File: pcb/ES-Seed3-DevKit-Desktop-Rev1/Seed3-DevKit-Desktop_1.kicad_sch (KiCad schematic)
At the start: 56 parts, among them J7 USB4110GFA, U12 CD4051B, U14 USBLC6-2SC6, U2 MCP6002-xSN, U4 4021, U5 4021, U6 MCP6002-xSN, U9 MCP6002-xSN

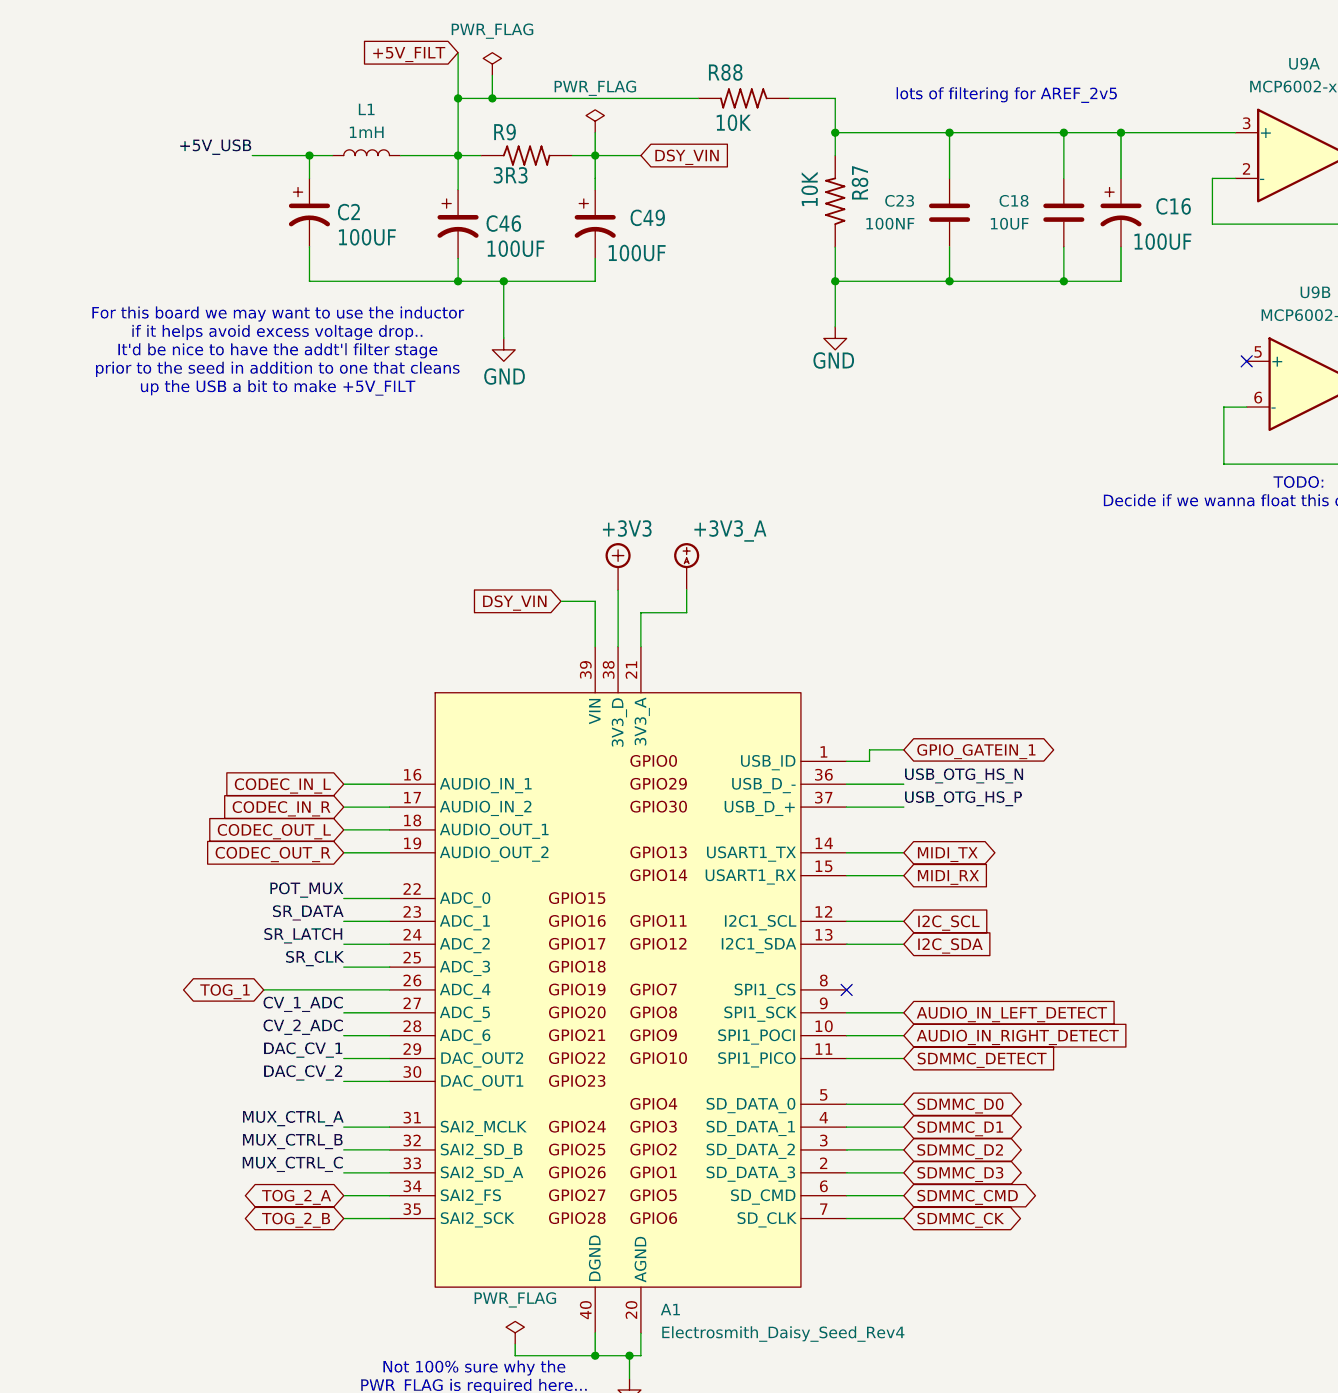
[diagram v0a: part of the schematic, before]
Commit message: routed, productions mats, etc.
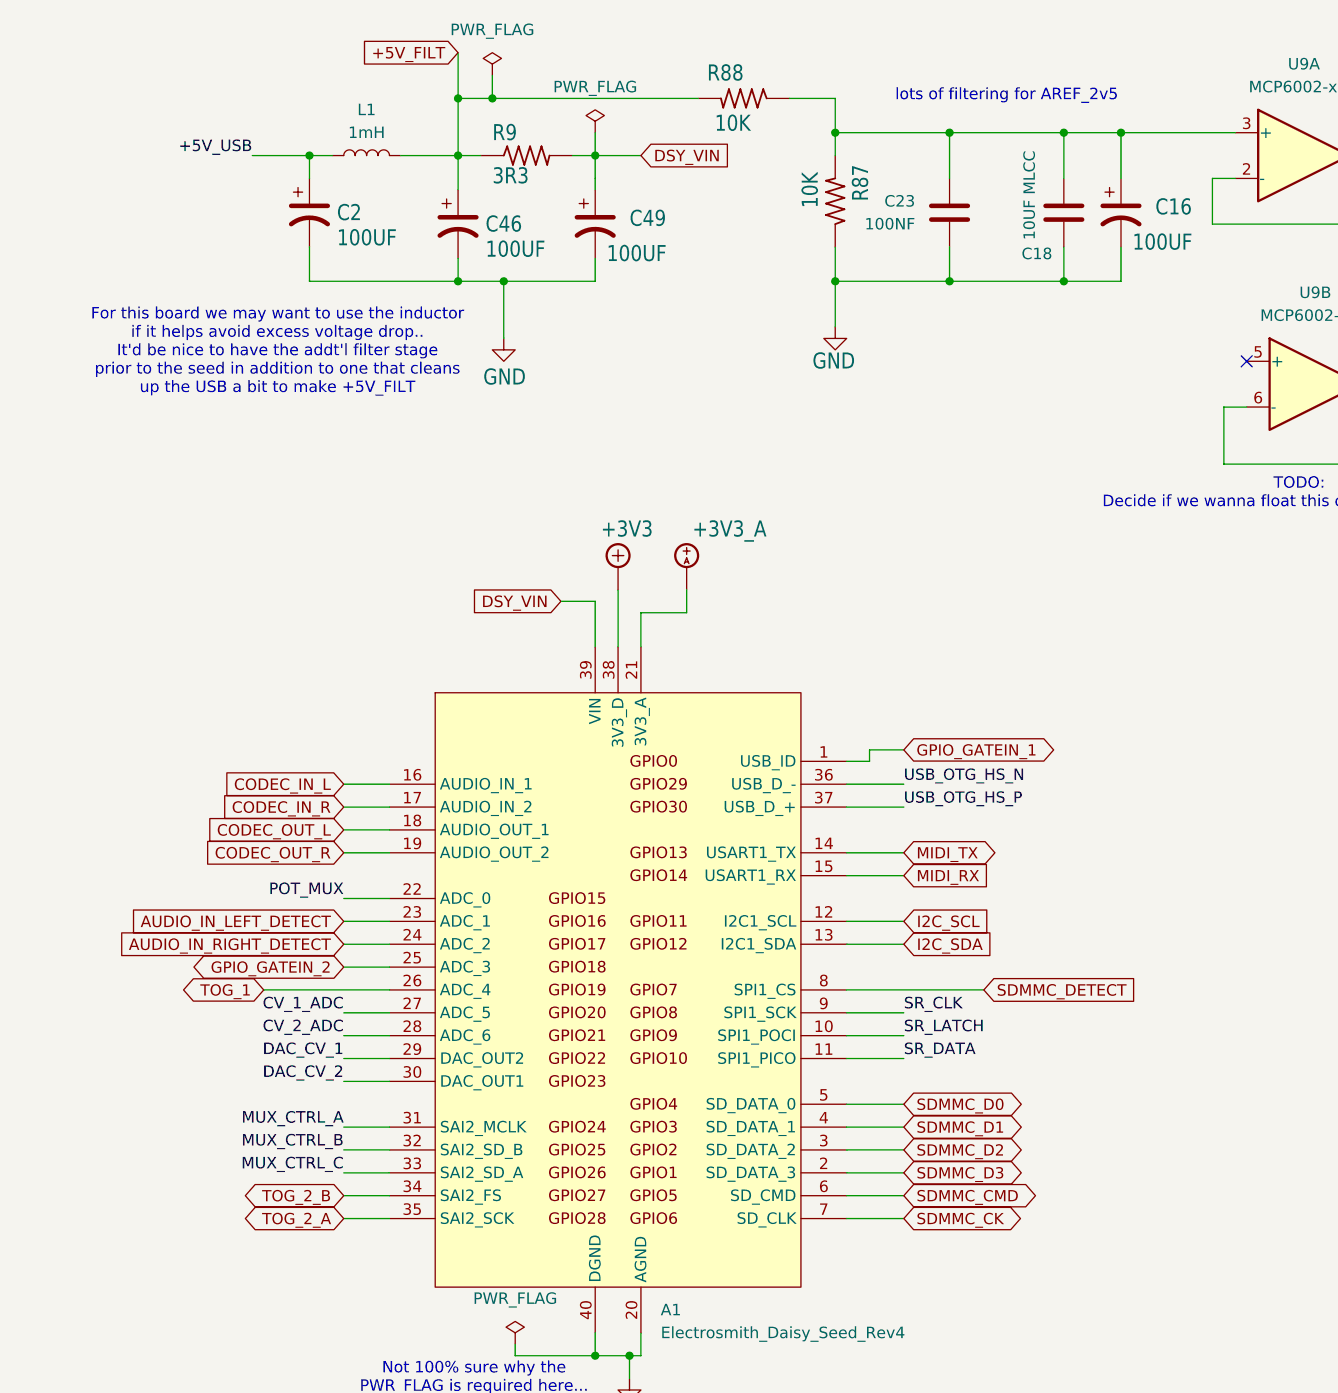
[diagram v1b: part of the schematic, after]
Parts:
- C18: value 10UF -> 10UF MLCC
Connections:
- net AUDIO_IN_LEFT_DETECT: now also A1.23 (ADC_1); no longer A1.9 (SPI1_SCK)
- net AUDIO_IN_RIGHT_DETECT: now also A1.24 (ADC_2); no longer A1.10 (SPI1_POCI)
- net SDMMC_DETECT: now also A1.8 (SPI1_CS); no longer A1.11 (SPI1_PICO)
- net SR_CLK: now also A1.9 (SPI1_SCK); no longer A1.25 (ADC_3)
- net SR_DATA: now also A1.11 (SPI1_PICO); no longer A1.23 (ADC_1)
- net SR_LATCH: now also A1.10 (SPI1_POCI); no longer A1.24 (ADC_2)
- net TOG_2_A: now also A1.35 (SAI2_SCK); no longer A1.34 (SAI2_FS)
- net TOG_2_B: now also A1.34 (SAI2_FS); no longer A1.35 (SAI2_SCK)
- new net GPIO_GATEIN_2: A1.25 (ADC_3)
- no-connect marks 17 -> 16
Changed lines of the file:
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@@
 	)
 	(no_connect
-		(at 87.63 109.22)
-	)
-	(no_connect
 		(at 266.7 175.26)
 	)
@@
 	(wire
 		(pts
+			(xy 87.63 109.22) (xy 102.87 109.22)
+		)
+		(stroke
+			(width 0)
+			(type default)
+		)
+	)
+	(wire
+		(pts
 			(xy 59.69 27.94) (xy 59.69 30.48)
 		)
@@
 	(wire
 		(pts
-			(xy 201.93 135.89) (xy 212.09 135.89)
+			(xy 31.75 106.68) (xy 36.83 106.68)
 		)
 		(stroke
@@
 	(wire
 		(pts
-			(xy 382.27 35.56) (xy 382.27 38.1)
+			(xy 201.93 135.89) (xy 212.09 135.89)
 		)
 		(stroke
@@
 	(wire
 		(pts
-			(xy 69.85 64.77) (xy 69.85 67.31)
+			(xy 382.27 35.56) (xy 382.27 38.1)
 		)
 		(stroke
@@
 	(wire
 		(pts
-			(xy 389.89 252.73) (xy 394.97 252.73)
+			(xy 69.85 64.77) (xy 69.85 67.31)
 		)
 		(stroke
@@
 	(wire
 		(pts
-			(xy 87.63 116.84) (xy 93.98 116.84)
+			(xy 389.89 252.73) (xy 394.97 252.73)
 		)
 		(stroke
@@
 	(wire
 		(pts
-			(xy 187.96 135.89) (xy 191.77 135.89)
+			(xy 87.63 116.84) (xy 93.98 116.84)
 		)
 		(stroke
@@
 	(wire
 		(pts
-			(xy 316.23 16.51) (xy 316.23 24.13)
+			(xy 187.96 135.89) (xy 191.77 135.89)
 		)
 		(stroke
@@
 	(wire
 		(pts
-			(xy 31.75 106.68) (xy 36.83 106.68)
+			(xy 316.23 16.51) (xy 316.23 24.13)
 		)
 		(stroke
@@
 	)
 	(label "SR_LATCH"
-		(at 31.75 104.14 180)
+		(at 93.98 114.3 0)
 		(effects
 			(font
 				(size 1.27 1.27)
 			)
-			(justify right bottom)
+			(justify left bottom)
 		)
 	)
@@
 		)
 	)
-	(label "SR_CLK"
-		(at 31.75 106.68 180)
-		(effects
-			(font
-				(size 1.27 1.27)
-			)
-			(justify right bottom)
-		)
-	)
 	(label "MUX_CTRL_A"
 		(at 31.75 124.46 180)
@@
 		)
 	)
+	(label "SR_CLK"
+		(at 93.98 111.76 0)
+		(effects
+			(font
+				(size 1.27 1.27)
+			)
+			(justify left bottom)
+		)
+	)
 	(label "SR_DATA"
-		(at 31.75 101.6 180)
+		(at 93.98 116.84 0)
 		(effects
 			(font
 				(size 1.27 1.27)
 			)
-			(justify right bottom)
+			(justify left bottom)
 		)
 	)
@@
 	(global_label "AUDIO_IN_LEFT_DETECT"
 		(shape input)
-		(at 93.98 111.76 0)
+		(at 31.75 101.6 180)
 		(fields_autoplaced yes)
 		(effects
@@
 				(size 1.27 1.27)
 			)
-			(justify left)
+			(justify right)
 		)
 		(property "Intersheetrefs" "${INTERSHEET_REFS}"
-			(at 118.4342 111.76 0)
+			(at 7.2958 101.6 0)
 			(effects
 				(font
 					(size 1.27 1.27)
 				)
-				(justify left)
+				(justify right)
 				(hide yes)
 			)
@@
 	(global_label "SDMMC_DETECT"
 		(shape input)
-		(at 93.98 116.84 0)
+		(at 102.87 109.22 0)
 		(fields_autoplaced yes)
 		(effects
@@
 		)
 		(property "Intersheetrefs" "${INTERSHEET_REFS}"
-			(at 111.3583 116.84 0)
+			(at 120.2483 109.22 0)
 			(effects
 				(font
@@
 		)
 	)
+	(global_label "GPIO_GATEIN_2"
+		(shape bidirectional)
+		(at 31.75 106.68 180)
+		(fields_autoplaced yes)
+		(effects
+			(font
+				(size 1.2446 1.2446)
+			)
+			(justify right)
+		)
+		(property "Intersheetrefs" "${INTERSHEET_REFS}"
+			(at 13.9857 106.68 0)
+			(effects
+				(font
+					(size 1.27 1.27)
+				)
+				(justify right)
+				(hide yes)
+			)
+		)
+	)
 	(global_label "MIDI_RX"
 		(shape input)
@@
 	(global_label "TOG_2_B"
 		(shape bidirectional)
-		(at 31.75 134.62 180)
+		(at 31.75 132.08 180)
 		(fields_autoplaced yes)
 		(effects
@@
 		)
 		(property "Intersheetrefs" "${INTERSHEET_REFS}"
-			(at 19.9125 134.62 0)
+			(at 20.0903 132.08 0)
 			(effects
 				(font
@@
 	(global_label "AUDIO_IN_RIGHT_DETECT"
 		(shape input)
-		(at 93.98 114.3 0)
+		(at 31.75 104.14 180)
 		(fields_autoplaced yes)
 		(effects
@@
 				(size 1.27 1.27)
 			)
-			(justify left)
+			(justify right)
 		)
 		(property "Intersheetrefs" "${INTERSHEET_REFS}"
-			(at 119.6438 114.3 0)
+			(at 6.0862 104.14 0)
 			(effects
 				(font
 					(size 1.27 1.27)
 				)
-				(justify left)
+				(justify right)
 				(hide yes)
 			)
@@
 	(global_label "TOG_2_A"
 		(shape bidirectional)
-		(at 31.75 132.08 180)
+		(at 31.75 134.62 180)
 		(fields_autoplaced yes)
 		(effects
@@
 		)
 		(property "Intersheetrefs" "${INTERSHEET_REFS}"
-			(at 20.0903 132.08 0)
+			(at 19.9125 134.62 0)
 			(effects
 				(font
@@
 		(dnp no)
 		(property "Reference" "C18"
-			(at 107.95 21.5899 0)
+			(at 110.49 27.432 0)
 			(effects
 				(font
@@
 			)
 		)
-		(property "Value" "10UF"
-			(at 107.95 24.1299 0)
+		(property "Value" "10UF MLCC"
+			(at 107.95 25.908 90)
 			(effects
 				(font
